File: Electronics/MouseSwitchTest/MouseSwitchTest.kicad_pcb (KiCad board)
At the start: 2 copper layers, 20.3 x 19.1 mm, 4 parts

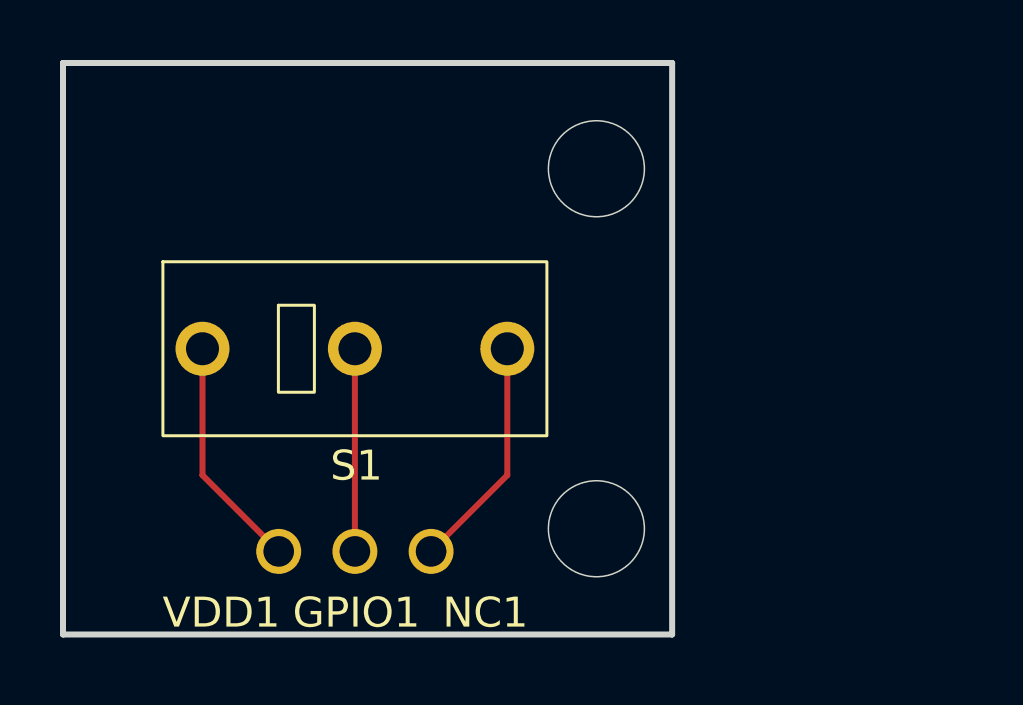
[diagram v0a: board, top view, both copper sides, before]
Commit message: updated the middle click pcb
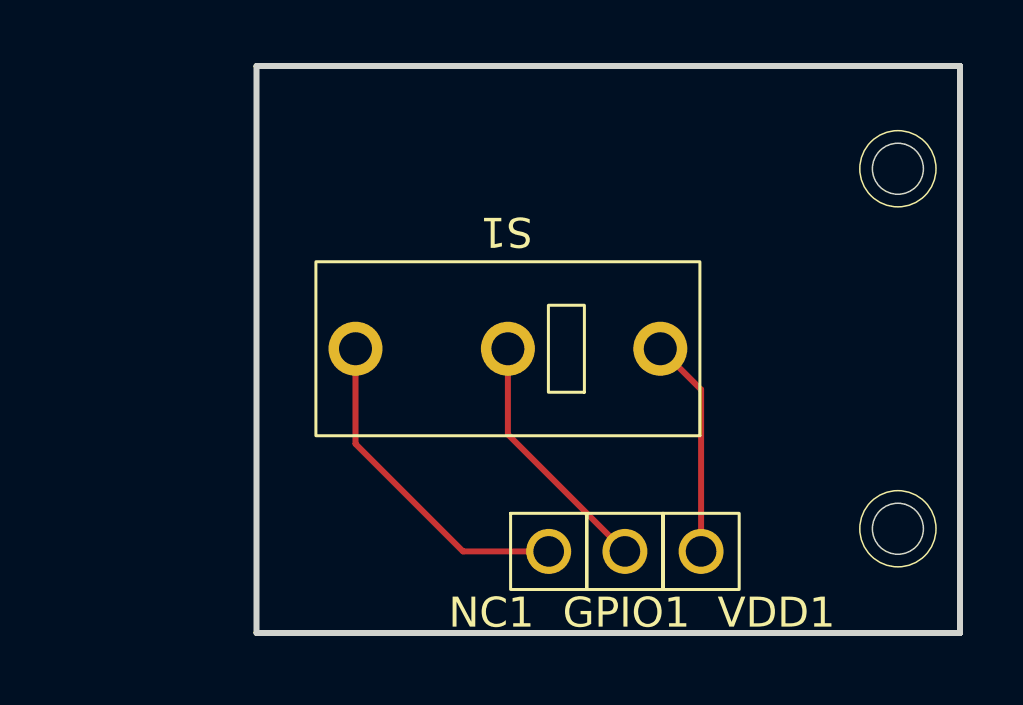
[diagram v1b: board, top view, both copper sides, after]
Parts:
- moved VDD1 14.1 mm to (13.5, 6.76)
- moved GPIO1 9.00 mm to (10.9, 6.76)
- moved S1 5.10 mm to (7.05, 0.00), turned to 180 degrees
- moved NC1 3.92 mm to (8.41, 6.76)
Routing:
- net Net-(NC1-Pin): track 7.81 -> 11.1 mm
- net Net-(GPIO1-Pin): track 6.76 -> 8.37 mm
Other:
- board size 20.3 x 19.1 mm -> 23.5 x 18.9 mm
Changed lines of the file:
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@@
 	(footprint "BardBarian_Footprints:Header"
 		(layer "F.Cu")
-		(at 4.49 6.7554)
+		(at 8.41 6.7554)
 		(property "Reference" "NC1"
-			(at 1.81 2.0446 0)
+			(at -1.91 2.0446 0)
 			(unlocked yes)
 			(layer "F.SilkS")
@@
 			)
 		)
-		(sheetname "Root")
-		(sheetfile "MouseSwitchTest.kicad_sch")
 		(attr through_hole)
 		(fp_rect
@@
 			)
 			(fill none)
+			(layer "F.SilkS")
+		)
+		(fp_rect
+			(start -1.27 -1.27)
+			(end 1.27 1.27)
+			(stroke
+				(width 0.1)
+				(type default)
+			)
+			(fill none)
 			(layer "Dwgs.User")
 		)
 		(fp_text user "${REFERENCE}"
-			(at 1.81 2.0446 0)
+			(at -1.91 2.0446 0)
 			(unlocked yes)
 			(layer "F.Fab")
@@
 	(footprint "BardBarian_Footprints:Header"
 		(layer "F.Cu")
-		(at -0.59 6.7554)
+		(at 13.49 6.7554)
 		(property "Reference" "VDD1"
-			(at -1.91 2.0446 0)
+			(at 2.51 2.0446 0)
 			(unlocked yes)
 			(layer "F.SilkS")
@@
 			)
 		)
-		(sheetname "Root")
-		(sheetfile "MouseSwitchTest.kicad_sch")
 		(attr through_hole)
 		(fp_rect
@@
 			)
 			(fill none)
+			(layer "F.SilkS")
+		)
+		(fp_rect
+			(start -1.27 -1.27)
+			(end 1.27 1.27)
+			(stroke
+				(width 0.1)
+				(type default)
+			)
+			(fill none)
 			(layer "Dwgs.User")
 		)
 		(fp_text user "${REFERENCE}"
-			(at -1.91 2.0446 0)
+			(at 2.51 2.0446 0)
 			(unlocked yes)
 			(layer "F.Fab")
@@
 	(footprint "BardBarian_Footprints:Header"
 		(layer "F.Cu")
-		(at 1.95 6.7554)
+		(at 10.95 6.7554)
 		(property "Reference" "GPIO1"
 			(at 0.05 2.0446 0)
@@
 			)
 		)
-		(sheetname "Root")
-		(sheetfile "MouseSwitchTest.kicad_sch")
 		(attr through_hole)
+		(fp_rect
+			(start -1.27 -1.27)
+			(end 1.27 1.27)
+			(stroke
+				(width 0.1)
+				(type default)
+			)
+			(fill none)
+			(layer "F.SilkS")
+		)
 		(fp_rect
 			(start -1.27 -1.27)
@@
 	(footprint "BardBarian_Footprints:Kailh GM 4.0 Red CMI126601D01"
 		(layer "F.Cu")
-		(at 1.95 0)
+		(at 7.05 0 180)
 		(property "Reference" "S1"
-			(at 0.05 3.9 0)
+			(at 0.05 3.9 180)
 			(unlocked yes)
 			(layer "F.SilkS")
@@
 		)
 		(property "Value" "~"
-			(at 0 1 0)
+			(at 0 1 180)
 			(unlocked yes)
 			(layer "F.Fab")
@@
 		)
 		(property "Footprint" "BardBarian_Footprints:Kailh GM 4.0 Red CMI126601D01"
-			(at 0 0 0)
+			(at 0 0 180)
 			(unlocked yes)
 			(layer "F.Fab")
@@
 		)
 		(property "Datasheet" ""
-			(at 0 0 0)
+			(at 0 0 180)
 			(unlocked yes)
 			(layer "F.Fab")
@@
 		)
 		(property "Description" ""
-			(at 0 0 0)
-			(unlocked yes)
-			(layer "F.Fab")
-			(hide yes)
-			(effects
-				(font
-					(size 1 1)
-					(thickness 0.15)
-				)
-			)
-		)
-		(sheetname "Root")
-		(sheetfile "MouseSwitchTest.kicad_sch")
+			(at 0 0 180)
+			(unlocked yes)
+			(layer "F.Fab")
+			(hide yes)
+			(effects
+				(font
+					(size 1 1)
+					(thickness 0.15)
+				)
+			)
+		)
 		(attr through_hole)
+		(fp_rect
+			(start -2.55 -1.45)
+			(end -1.35 1.45)
+			(stroke
+				(width 0.1)
+				(type default)
+			)
+			(fill none)
+			(layer "F.SilkS")
+		)
 		(fp_rect
 			(start -6.4 -2.9)
@@
 			)
 			(fill none)
-			(layer "F.SilkS")
+			(layer "Dwgs.User")
 		)
 		(fp_rect
@@
 			(layer "Dwgs.User")
 		)
-		(fp_rect
-			(start -2.55 -1.45)
-			(end -1.35 1.45)
-			(stroke
-				(width 0.1)
-				(type default)
-			)
-			(fill none)
-			(layer "Dwgs.User")
-		)
 		(fp_text user "${REFERENCE}"
-			(at 0.05 3.9 0)
+			(at 0.05 3.9 180)
 			(unlocked yes)
 			(layer "F.Fab")
@@
 		)
 		(pad "1" thru_hole circle
-			(at -5.08 0)
+			(at -5.08 0 180)
 			(size 1.8 1.8)
 			(drill 1.1)
@@
 		)
 		(pad "2" thru_hole circle
-			(at 0 0)
+			(at 0 0 180)
 			(size 1.8 1.8)
 			(drill 1.1)
@@
 		)
 		(pad "3" thru_hole circle
-			(at 5.08 0)
+			(at 5.08 0 180)
 			(size 1.8 1.8)
 			(drill 1.1)
@@
 	)
 	(gr_circle
-		(center 10 6)
-		(end 11.6 6)
+		(center 20.05 -6)
+		(end 21.32 -6)
 		(stroke
 			(width 0.05)
@@
 		)
 		(fill none)
-		(layer "Edge.Cuts")
+		(layer "F.SilkS")
 	)
 	(gr_circle
-		(center 10 -6)
-		(end 11.6 -6)
+		(center 20.05 6)
+		(end 21.32 6)
 		(stroke
 			(width 0.05)
@@
 		)
 		(fill none)
+		(layer "F.SilkS")
+	)
+	(gr_circle
+		(center 20.05 6)
+		(end 20.9 6)
+		(stroke
+			(width 0.05)
+			(type default)
+		)
+		(fill none)
 		(layer "Edge.Cuts")
 	)
+	(gr_circle
+		(center 20.05 -6)
+		(end 20.9 -6)
+		(stroke
+			(width 0.05)
+			(type default)
+		)
+		(fill none)
+		(layer "Edge.Cuts")
+	)
 	(gr_rect
-		(start -7.78 -9.525)
-		(end 12.525 9.525)
+		(start -1.33 9.475)
+		(end 22.12 -9.425)
 		(stroke
 			(width 0.2)
@@
 	)
 	(segment
-		(start 1.95 0)
-		(end 1.95 6.7554)
+		(start 7.05 0)
+		(end 7.05 2.8554)
 		(width 0.2)
 		(layer "F.Cu")
@@
 	)
 	(segment
-		(start -3.13 4.2154)
-		(end -0.59 6.7554)
+		(start 7.05 2.8554)
+		(end 10.95 6.7554)
+		(width 0.2)
+		(layer "F.Cu")
+		(net 1)
+	)
+	(segment
+		(start 13.49 1.36)
+		(end 13.49 6.7554)
 		(width 0.2)
 		(layer "F.Cu")
@@
 	)
 	(segment
-		(start -3.13 0)
-		(end -3.13 4.2154)
+		(start 12.13 0)
+		(end 13.49 1.36)
 		(width 0.2)
 		(layer "F.Cu")
@@
 	)
 	(segment
-		(start 7.03 0)
-		(end 7.03 4.2154)
+		(start 1.97 3.17)
+		(end 5.5554 6.7554)
 		(width 0.2)
 		(layer "F.Cu")
@@
 	)
 	(segment
-		(start 7.03 4.2154)
-		(end 4.49 6.7554)
-		(width 0.2)
-		(layer "F.Cu")
+		(start 5.5554 6.7554)
+		(end 8.41 6.7554)
+		(width 0.2)
+		(layer "F.Cu")
+		(net 3)
+	)
+	(segment
+		(start 1.97 0)
+		(end 1.97 3.17)
+		(width 0.2)
+		(layer "F.Cu")
